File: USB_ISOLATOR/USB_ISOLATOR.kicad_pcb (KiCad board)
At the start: 4 copper layers, 45 x 29 mm, 37 parts, among them J1 USB_A, J3 Conn_01x02, Q1 MMBT3904, U1 ADUM4160, U2 EL814, U4 LMV321, U5 SRV05-4, U6 SRV05-4

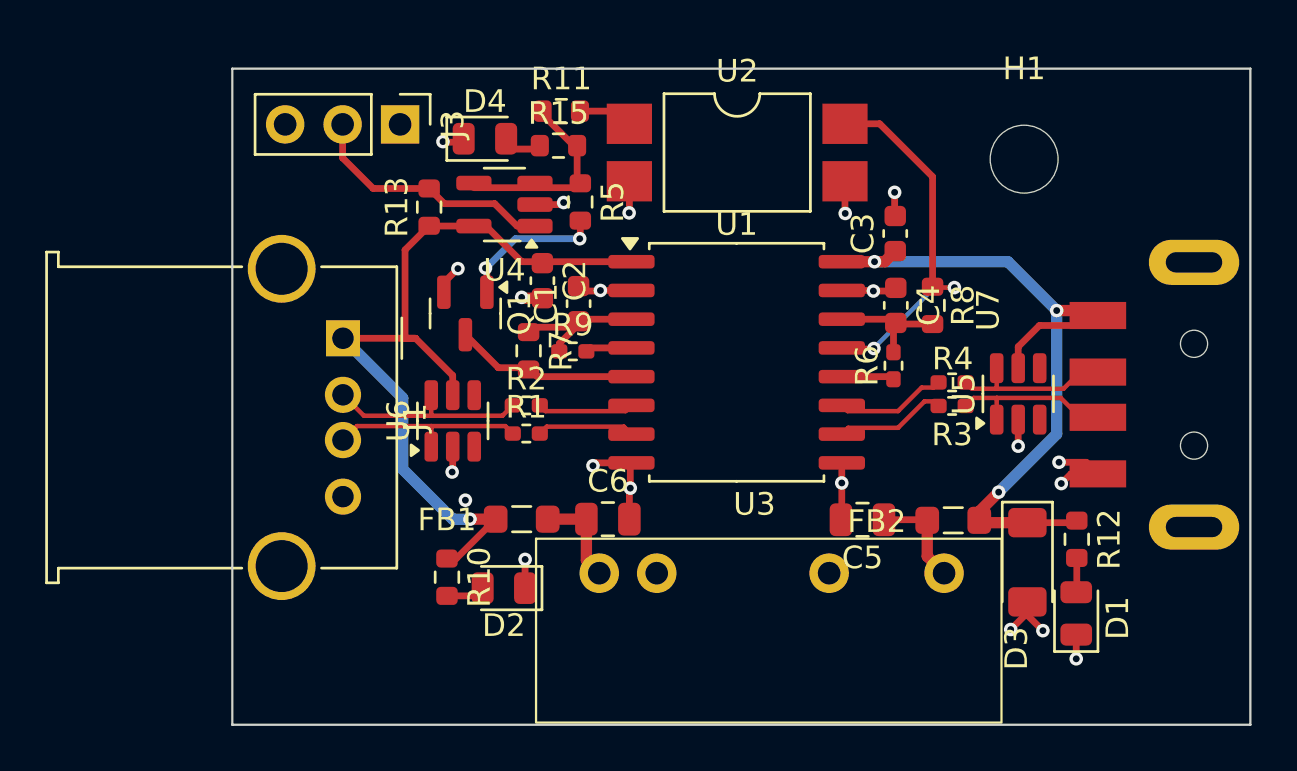
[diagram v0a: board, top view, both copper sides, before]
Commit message: g
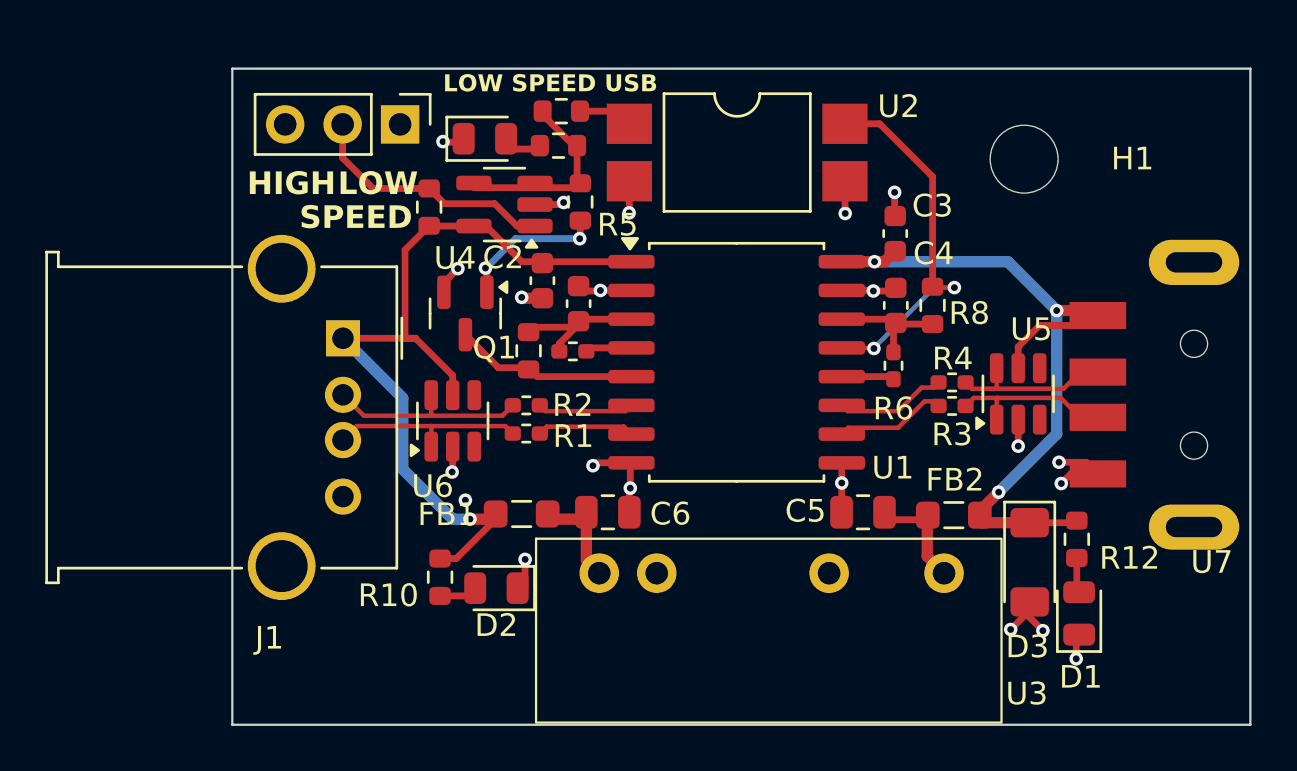
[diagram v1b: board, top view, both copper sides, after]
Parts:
- moved C5 0.33 mm to (147.9, 111.6)
- moved D2 0.33 mm to (131.7, 115.0)
- moved C6 0.30 mm to (136.6, 111.6)
- moved R10 0.30 mm to (129.2, 114.5)
- moved FB2 0.23 mm to (151.9, 111.7)
- moved FB1 0.23 mm to (132.8, 111.7)
- moved D1 0.13 mm to (157.4, 116.1)
- moved D3 0.10 mm to (155.2, 113.8)
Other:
- board text added: "HIGH"
- board text added: "LOW"
- board text added: "LOW SPEED USB"
- board text added: "SPEED"
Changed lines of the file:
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@@
 		(tags "capacitor")
 		(property "Reference" "C1"
-			(at 0 -1.43 -90)
+			(at 0 -1.43 270)
 			(layer "F.SilkS")
+			(hide yes)
 			(effects
 				(font
@@
 	(footprint "Capacitor_SMD:C_0805_2012Metric"
 		(layer "F.Cu")
-		(at 136.6012 111.9124)
+		(at 136.6012 111.6076)
 		(descr "Capacitor SMD 0805 (2012 Metric), square (rectangular) end terminal, IPC_7351 nominal, (Body size source: IPC-SM-782 page 76, https://www.pcb-3d.com/wordpress/wp-content/uploads/ipc-sm-782a_amendment_1_and_2.pdf, https://docs.google.com/spreadsheets/d/1BsfQQcO9C6DZCsRaXUlFlo91Tg2WpOkGARC1WS5S8t0/edit?usp=sharing), generated with kicad-footprint-generator")
 		(tags "capacitor")
 		(property "Reference" "C6"
-			(at 0 -1.68 0)
+			(at 2.7686 0.0762 0)
 			(layer "F.SilkS")
 			(effects
@@
 		(tags "SMD DIP DIL PDIP SMDIP 2.54mm 9.53mm 375mil")
 		(property "Reference" "U2"
-			(at 0 -3.6 0)
+			(at 7.1374 -2.032 0)
 			(layer "F.SilkS")
 			(effects
@@
 		(tags "SOT TO_SOT_SMD")
 		(property "Reference" "U6"
-			(at 0 -2.4 270)
+			(at -2.8956 -0.889 0)
 			(layer "F.SilkS")
 			(effects
@@
 		)
 		(property "Value" "SRV05-4"
-			(at 0 2.4 270)
+			(at 0 2.4 -90)
 			(layer "F.Fab")
 			(effects
@@
 		)
 		(fp_text user "${REFERENCE}"
-			(at 0 0 270)
+			(at 0 0 -90)
 			(layer "F.Fab")
 			(effects
@@
 		(tags "SOT TO_SOT_SMD")
 		(property "Reference" "U5"
-			(at 0 -2.4 270)
+			(at 2.8448 0.5842 0)
 			(layer "F.SilkS")
 			(effects
@@
 		)
 		(property "Value" "SRV05-4"
-			(at 0 2.4 270)
+			(at 0 2.4 -90)
 			(layer "F.Fab")
 			(effects
@@
 		)
 		(fp_text user "${REFERENCE}"
-			(at 0 0 270)
+			(at 0 0 -90)
 			(layer "F.Fab")
 			(effects
@@
 		(tags "SOIC SO")
 		(property "Reference" "U1"
-			(at 0 -6.1 0)
+			(at 6.9088 4.6736 0)
 			(layer "F.SilkS")
 			(effects
@@
 		(tags "Through hole pin header THT 1x03 2.54mm single row")
 		(property "Reference" "J3"
-			(at 0 -2.33 -90)
+			(at -1.1684 -2.682 0)
 			(layer "F.SilkS")
+			(hide yes)
 			(effects
 				(font
@@
 		(tags "capacitor")
 		(property "Reference" "C4"
-			(at 0 1.4478 -90)
+			(at 2.286 1.6764 0)
 			(layer "F.SilkS")
 			(effects
@@
 			(at 0 -1.43 0)
 			(layer "F.SilkS")
+			(hide yes)
 			(effects
 				(font
@@
 	(footprint "Capacitor_SMD:C_0805_2012Metric"
 		(layer "F.Cu")
-		(at 147.8534 111.9378 180)
+		(at 147.8788 111.6076 180)
 		(descr "Capacitor SMD 0805 (2012 Metric), square (rectangular) end terminal, IPC_7351 nominal, (Body size source: IPC-SM-782 page 76, https://www.pcb-3d.com/wordpress/wp-content/uploads/ipc-sm-782a_amendment_1_and_2.pdf, https://docs.google.com/spreadsheets/d/1BsfQQcO9C6DZCsRaXUlFlo91Tg2WpOkGARC1WS5S8t0/edit?usp=sharing), generated with kicad-footprint-generator")
 		(tags "capacitor")
 		(property "Reference" "C5"
-			(at 0 -1.68 180)
+			(at 2.54 0.0508 180)
 			(layer "F.SilkS")
 			(effects
@@
 		(tags "SOT TO_SOT_SMD")
 		(property "Reference" "Q1"
-			(at 0 -2.4 90)
+			(at 1.5217 -1.2954 180)
 			(layer "F.SilkS")
 			(effects
@@
 		(tags "resistor")
 		(property "Reference" "R13"
-			(at 0 -1.43 -90)
+			(at -1.905 -2.1844 0)
 			(layer "F.SilkS")
+			(hide yes)
 			(effects
 				(font
@@
 		(tags "resistor")
 		(property "Reference" "R7"
-			(at 0 -1.43 90)
+			(at 1.143 -1.6002 180)
 			(layer "F.SilkS")
+			(hide yes)
 			(effects
 				(font
@@
 	(footprint "Resistor_SMD:R_0603_1608Metric"
 		(layer "F.Cu")
-		(at 129.4892 114.4778 -90)
+		(at 129.1844 114.4778 -90)
 		(descr "Resistor SMD 0603 (1608 Metric), square (rectangular) end terminal, IPC_7351 nominal, (Body size source: IPC-SM-782 page 72, https://www.pcb-3d.com/wordpress/wp-content/uploads/ipc-sm-782a_amendment_1_and_2.pdf), generated with kicad-footprint-generator")
 		(tags "resistor")
 		(property "Reference" "R10"
-			(at 0 -1.43 90)
+			(at 0.8128 2.286 180)
 			(layer "F.SilkS")
 			(effects
@@
 		(tags "resistor")
 		(property "Reference" "R12"
-			(at 0 -1.43 90)
+			(at 0.8382 -2.3368 180)
 			(layer "F.SilkS")
 			(effects
@@
 		(tags "resistor")
 		(property "Reference" "R8"
-			(at 0 1.3462 -90)
+			(at -0.3556 1.6256 0)
 			(layer "F.SilkS")
 			(effects
@@
 		(tags "capacitor")
 		(property "Reference" "C2"
-			(at 0 -1.43 90)
+			(at -1.016 1.7272 180)
 			(layer "F.SilkS")
 			(effects
@@
 		(tags "resistor handsolder")
 		(property "Reference" "R1"
-			(at 0 -1.17 0)
+			(at 2.0828 0.127 0)
 			(layer "F.SilkS")
 			(effects
@@
 		(tags "resistor")
 		(property "Reference" "R5"
-			(at 0 -1.43 90)
+			(at 1.016 -1.651 0)
 			(layer "F.SilkS")
 			(effects
@@
 		(at 162.5092 108.6612 90)
 		(property "Reference" "U7"
-			(at 6 -9.1 90)
+			(at -5.1562 0.7874 0)
 			(unlocked yes)
 			(layer "F.SilkS")
@@
 		(tags "USB_A Female Connector receptacle")
 		(property "Reference" "J1"
-			(at 3.5 -3.19 90)
+			(at 13.2536 3.2518 180)
 			(layer "F.SilkS")
 			(effects
@@
 	(footprint "LED_SMD:LED_0805_2012Metric"
 		(layer "F.Cu")
-		(at 157.3022 116.078 90)
+		(at 157.4292 116.078 90)
 		(descr "LED SMD 0805 (2012 Metric), square (rectangular) end terminal, IPC_7351 nominal, (Body size source: https://docs.google.com/spreadsheets/d/1BsfQQcO9C6DZCsRaXUlFlo91Tg2WpOkGARC1WS5S8t0/edit?usp=sharing), generated with kicad-footprint-generator")
 		(tags "LED")
 		(property "Reference" "D1"
-			(at -0.2032 1.8288 -90)
+			(at -2.8194 0.0762 0)
 			(layer "F.SilkS")
 			(effects
@@
 	(footprint "Inductor_SMD:L_0805_2012Metric_Pad1.05x1.20mm_HandSolder"
 		(layer "F.Cu")
-		(at 132.7912 111.9124)
+		(at 132.7912 111.6838)
 		(descr "Inductor SMD 0805 (2012 Metric), square (rectangular) end terminal, IPC_7351 nominal with elongated pad for handsoldering. (Body size source: IPC-SM-782 page 80, https://www.pcb-3d.com/wordpress/wp-content/uploads/ipc-sm-782a_amendment_1_and_2.pdf), generated with kicad-footprint-generator")
 		(tags "inductor handsolder")
@@
 		(tags "SOT-23-5 hand-soldering")
 		(property "Reference" "U4"
-			(at 0 -2.9 180)
+			(at 2.1844 -2.3739 180)
 			(layer "F.SilkS")
 			(effects
@@
 	(footprint "Inductor_SMD:L_0805_2012Metric_Pad1.05x1.20mm_HandSolder"
 		(layer "F.Cu")
-		(at 151.8666 111.9632)
+		(at 151.892 111.7346)
 		(descr "Inductor SMD 0805 (2012 Metric), square (rectangular) end terminal, IPC_7351 nominal with elongated pad for handsoldering. (Body size source: IPC-SM-782 page 80, https://www.pcb-3d.com/wordpress/wp-content/uploads/ipc-sm-782a_amendment_1_and_2.pdf), generated with kicad-footprint-generator")
 		(tags "inductor handsolder")
 		(property "Reference" "FB2"
-			(at -3.3782 0.0508 0)
+			(at 0.0508 -1.5494 0)
 			(layer "F.SilkS")
 			(effects
@@
 		(tags "LED")
 		(property "Reference" "D4"
-			(at 0 -1.65 0)
+			(at 0.635 -1.65 0)
 			(layer "F.SilkS")
+			(hide yes)
 			(effects
 				(font
@@
 	(footprint "LED_SMD:LED_0805_2012Metric"
 		(layer "F.Cu")
-		(at 132.0038 114.9604 180)
+		(at 131.6736 114.9604 180)
 		(descr "LED SMD 0805 (2012 Metric), square (rectangular) end terminal, IPC_7351 nominal, (Body size source: https://docs.google.com/spreadsheets/d/1BsfQQcO9C6DZCsRaXUlFlo91Tg2WpOkGARC1WS5S8t0/edit?usp=sharing), generated with kicad-footprint-generator")
 		(tags "LED")
@@
 		(tags "mounting hole 3mm no annular")
 		(property "Reference" "H1"
-			(at 0 -4 0)
+			(at 4.7914 -0.0134 0)
 			(layer "F.SilkS")
 			(effects
@@
 		(tags "resistor handsolder")
 		(property "Reference" "R6"
-			(at 0 -1.17 -90)
+			(at -1.905 0 0)
 			(layer "F.SilkS")
 			(effects
@@
 			(at 0 -1.43 0)
 			(layer "F.SilkS")
+			(hide yes)
 			(effects
 				(font
@@
 		(at 136.2202 114.3)
 		(property "Reference" "U3"
-			(at 6.858 -3.048 0)
+			(at 18.8976 5.334 0)
 			(unlocked yes)
 			(layer "F.SilkS")
@@
 			(at 0 -1.17 0)
 			(layer "F.SilkS")
+			(hide yes)
 			(effects
 				(font
@@
 	(footprint "Diode_SMD:D_MiniMELF"
 		(layer "F.Cu")
-		(at 155.1432 113.8174 -90)
+		(at 155.2448 113.8174 -90)
 		(descr "Diode Mini-MELF (SOD-80)")
 		(tags "Diode Mini-MELF (SOD-80)")
 		(property "Reference" "D3"
-			(at 3.81 0.4826 90)
+			(at 3.7338 0.1016 180)
 			(layer "F.SilkS")
 			(effects
@@
 		(tags "resistor handsolder")
 		(property "Reference" "R2"
-			(at 0 -1.17 0)
+			(at 2.0574 0 0)
 			(layer "F.SilkS")
 			(effects
@@
 		(tags "capacitor")
 		(property "Reference" "C3"
-			(at 0 -1.43 270)
+			(at 1.2192 1.651 0)
 			(layer "F.SilkS")
 			(effects
@@
 		)
 		(property "Value" "220n"
-			(at 0 1.43 270)
+			(at 0 1.43 -90)
 			(layer "F.Fab")
 			(effects
@@
 		)
 		(fp_text user "${REFERENCE}"
-			(at 0 0 270)
+			(at 0 0 -90)
 			(layer "F.Fab")
 			(effects
@@
 		(layer "Edge.Cuts")
 	)
+	(gr_text "LOW SPEED USB"
+		(at 129.3114 93.091 0)
+		(layer "F.SilkS" knockout)
+		(effects
+			(font
+				(size 0.75 0.75)
+				(thickness 0.13)
+				(bold yes)
+			)
+			(justify left bottom)
+		)
+	)
+	(gr_text "LOW"
+		(at 124.6632 97.663 0)
+		(layer "F.SilkS" knockout)
+		(effects
+			(font
+				(size 1 1)
+				(thickness 0.2)
+				(bold yes)
+			)
+			(justify left bottom)
+		)
+	)
+	(gr_text "SPEED"
+		(at 122.9614 99.1616 0)
+		(layer "F.SilkS" knockout)
+		(effects
+			(font
+				(size 1 1)
+				(thickness 0.2)
+				(bold yes)
+			)
+			(justify left bottom)
+		)
+	)
+	(gr_text "HIGH"
+		(at 120.65 97.663 0)
+		(layer "F.SilkS" knockout)
+		(effects
+			(font
+				(size 1 1)
+				(thickness 0.2)
+				(bold yes)
+			)
+			(justify left bottom)
+		)
+	)
 	(segment
